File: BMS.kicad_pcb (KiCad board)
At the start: 2 copper layers, 2 parts, among them U1 ATtiny824-SSU, U2 TLV61070ADBV

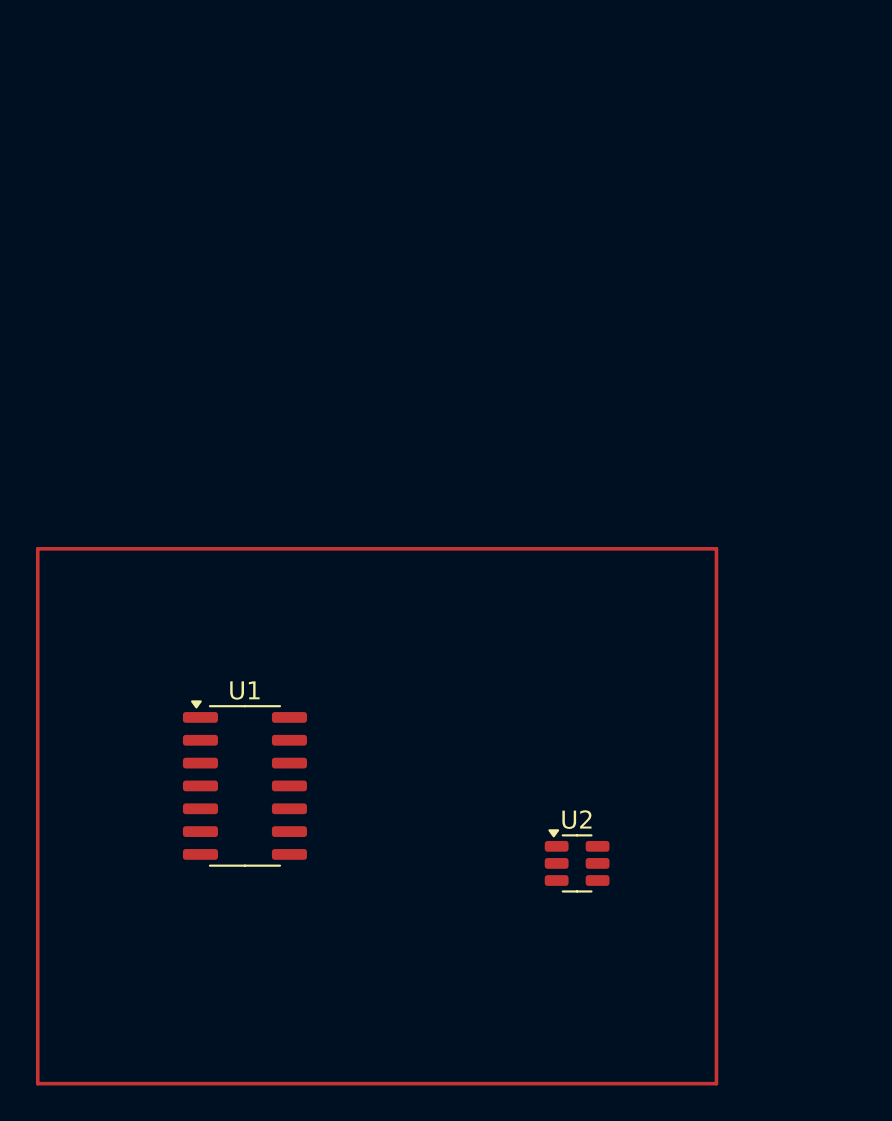
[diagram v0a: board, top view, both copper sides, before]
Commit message: Finished schematic
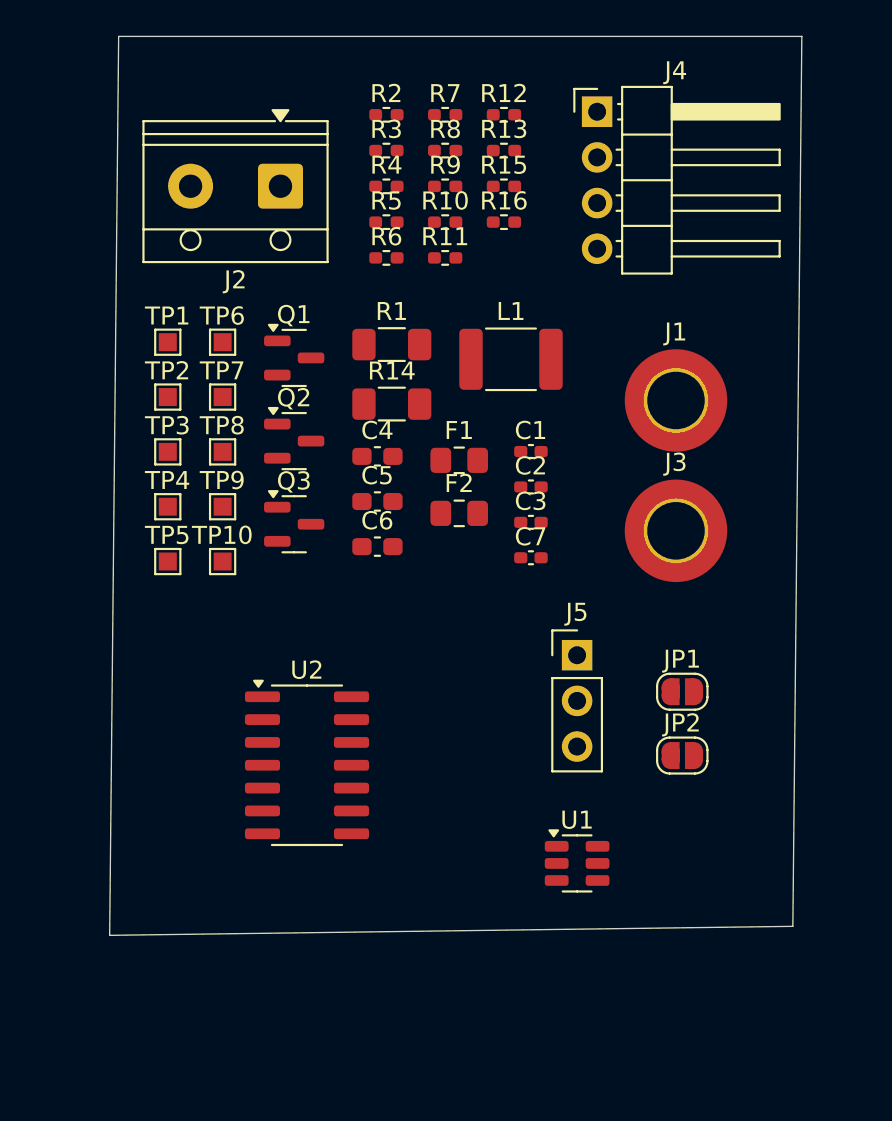
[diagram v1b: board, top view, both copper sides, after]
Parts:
- added C1: 100n, Capacitor_SMD:C_0402_1005Metric_Pad0.74x0.62mm_HandSolder, F.Cu at (150.4, 75.6)
- added C2: 100n, Capacitor_SMD:C_0402_1005Metric_Pad0.74x0.62mm_HandSolder, F.Cu at (150.4, 77.6)
- added C3: 100n, Capacitor_SMD:C_0402_1005Metric_Pad0.74x0.62mm_HandSolder, F.Cu at (150.4, 79.5)
- added C4: 10u, Capacitor_SMD:C_0603_1608Metric_Pad1.08x0.95mm_HandSolder, F.Cu at (141.9, 75.9)
- added C5: 10u, Capacitor_SMD:C_0603_1608Metric_Pad1.08x0.95mm_HandSolder, F.Cu at (141.9, 78.4)
- added C6: 10u, Capacitor_SMD:C_0603_1608Metric_Pad1.08x0.95mm_HandSolder, F.Cu at (141.9, 80.9)
- added C7: 270p, Capacitor_SMD:C_0402_1005Metric_Pad0.74x0.62mm_HandSolder, F.Cu at (150.4, 81.5)
- added F1: BSMD0805-110-6V, Fuse:Fuse_0805_2012Metric_Pad1.15x1.40mm_HandSolder, F.Cu at (146.4, 76.1)
- added F2: BSMD0805-110-6V, Fuse:Fuse_0805_2012Metric_Pad1.15x1.40mm_HandSolder, F.Cu at (146.4, 79.0)
- added J1: BATT+, MountingHole:MountingHole_3.2mm_M3_ISO7380_Pad_TopOnly, F.Cu at (158.5, 72.8)
- added J2: LOAD, TerminalBlock_RND:TerminalBlock_RND_205-00012_1x02_P5.00mm_Horizontal, F.Cu at (136.5, 60.8)
- added J3: BATT-, MountingHole:MountingHole_3.2mm_M3_ISO7380_Pad_TopOnly, F.Cu at (158.5, 80.0)
- added J4: QWIIC, Connector_PinHeader_2.54mm:PinHeader_1x04_P2.54mm_Horizontal, F.Cu at (154.1, 56.7)
- added J5: PROG, Connector_PinHeader_2.54mm:PinHeader_1x03_P2.54mm_Vertical, F.Cu at (153.0, 86.9)
- added JP1: MCU_VCC, Jumper:SolderJumper-2_P1.3mm_Open_RoundedPad1.0x1.5mm, F.Cu at (158.8, 89.0)
- added JP2: I2C_V, Jumper:SolderJumper-2_P1.3mm_Open_RoundedPad1.0x1.5mm, F.Cu at (158.8, 92.5)
- added L1: 2.2uH, Inductor_SMD:L_1812_4532Metric_Pad1.30x3.40mm_HandSolder, F.Cu at (149.3, 70.5)
- added Q1: SI2333, Package_TO_SOT_SMD:SOT-23, F.Cu at (137.3, 70.4)
- added Q2: SI2333, Package_TO_SOT_SMD:SOT-23, F.Cu at (137.3, 75.0)
- added Q3: SI2333, Package_TO_SOT_SMD:SOT-23, F.Cu at (137.3, 79.6)
- added R1: 0.1R, Resistor_SMD:R_1206_3216Metric_Pad1.30x1.75mm_HandSolder, F.Cu at (142.7, 69.6)
- added R10: 100k, Resistor_SMD:R_0402_1005Metric_Pad0.72x0.64mm_HandSolder, F.Cu at (145.7, 62.8)
- added R11: 120R, Resistor_SMD:R_0402_1005Metric_Pad0.72x0.64mm_HandSolder, F.Cu at (145.7, 64.8)
- added R12: 120R, Resistor_SMD:R_0402_1005Metric_Pad0.72x0.64mm_HandSolder, F.Cu at (148.9, 56.9)
- added R13: 1M, Resistor_SMD:R_0402_1005Metric_Pad0.72x0.64mm_HandSolder, F.Cu at (148.9, 58.9)
- added R14: 0.1R, Resistor_SMD:R_1206_3216Metric_Pad1.30x1.75mm_HandSolder, F.Cu at (142.7, 73.0)
- added R15: 120R, Resistor_SMD:R_0402_1005Metric_Pad0.72x0.64mm_HandSolder, F.Cu at (148.9, 60.8)
- added R16: 100k, Resistor_SMD:R_0402_1005Metric_Pad0.72x0.64mm_HandSolder, F.Cu at (148.9, 62.8)
- added R2: 1M, Resistor_SMD:R_0402_1005Metric_Pad0.72x0.64mm_HandSolder, F.Cu at (142.4, 56.9)
- added R3: 1M, Resistor_SMD:R_0402_1005Metric_Pad0.72x0.64mm_HandSolder, F.Cu at (142.4, 58.9)
- added R4: 1M, Resistor_SMD:R_0402_1005Metric_Pad0.72x0.64mm_HandSolder, F.Cu at (142.4, 60.8)
- added R5: 1M, Resistor_SMD:R_0402_1005Metric_Pad0.72x0.64mm_HandSolder, F.Cu at (142.4, 62.8)
- added R6: 1M, Resistor_SMD:R_0402_1005Metric_Pad0.72x0.64mm_HandSolder, F.Cu at (142.4, 64.8)
- added R7: 1M, Resistor_SMD:R_0402_1005Metric_Pad0.72x0.64mm_HandSolder, F.Cu at (145.7, 56.9)
- added R8: 1M, Resistor_SMD:R_0402_1005Metric_Pad0.72x0.64mm_HandSolder, F.Cu at (145.7, 58.9)
- added R9: 560k, Resistor_SMD:R_0402_1005Metric_Pad0.72x0.64mm_HandSolder, F.Cu at (145.7, 60.8)
- added TP1: TestPoint, TestPoint:TestPoint_Pad_1.0x1.0mm, F.Cu at (130.2, 69.5)
- added TP10: TestPoint, TestPoint:TestPoint_Pad_1.0x1.0mm, F.Cu at (133.3, 81.7)
- added TP2: TestPoint, TestPoint:TestPoint_Pad_1.0x1.0mm, F.Cu at (130.2, 72.6)
- added TP3: TestPoint, TestPoint:TestPoint_Pad_1.0x1.0mm, F.Cu at (130.2, 75.6)
- added TP4: TestPoint, TestPoint:TestPoint_Pad_1.0x1.0mm, F.Cu at (130.2, 78.7)
- added TP5: TestPoint, TestPoint:TestPoint_Pad_1.0x1.0mm, F.Cu at (130.2, 81.7)
- added TP6: TestPoint, TestPoint:TestPoint_Pad_1.0x1.0mm, F.Cu at (133.3, 69.5)
- added TP7: TestPoint, TestPoint:TestPoint_Pad_1.0x1.0mm, F.Cu at (133.3, 72.6)
- added TP8: TestPoint, TestPoint:TestPoint_Pad_1.0x1.0mm, F.Cu at (133.3, 75.6)
- added TP9: TestPoint, TestPoint:TestPoint_Pad_1.0x1.0mm, F.Cu at (133.3, 78.7)
- moved U2 3.64 mm to (138.0, 93.0)
- renumbered U2 to U1, U1 to U2
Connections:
- U1 pad 1: unconnected-(U2-SW-Pad1) -> Net-(U1-SW)
- U1 pad 2: unconnected-(U2-GND-Pad2) -> GND
- U1 pad 3: unconnected-(U2-EN-Pad3) -> Net-(JP1-B)
- U1 pad 4: unconnected-(U2-V_{FB}-Pad4) -> Net-(U1-V_{FB})
- U1 pad 5: unconnected-(U2-V_{OUT}-Pad5) -> VCC
- U1 pad 6: unconnected-(U2-V_{IN}-Pad6) -> Net-(JP1-B)
- U2 pad 1: unconnected-(U1-VCC-Pad1) -> VCC
- U2 pad 10: unconnected-(U1-~{RESET}/PA0-Pad10) -> UPDI
- U2 pad 11: unconnected-(U1-PA1-Pad11) -> ADC_SP
- U2 pad 12: unconnected-(U1-AIN2-Pad12) -> ADC_BATT
- U2 pad 13: unconnected-(U1-AIN3-Pad13) -> ADC_LOAD
- U2 pad 14: unconnected-(U1-GND-Pad14) -> GND
- U2 pad 2: unconnected-(U1-PA4-Pad2) -> CUTOFF
- U2 pad 3: unconnected-(U1-PA5-Pad3) -> Net-(U2-PA5)
- U2 pad 4: unconnected-(U1-AIN6-Pad4) -> ADC_LN
- U2 pad 5: unconnected-(U1-AIN7-Pad5) -> ADC_LP
- U2 pad 6: unconnected-(U1-RXD-Pad6) -> 3V3CUTOFF
- U2 pad 7: unconnected-(U1-TXD-Pad7) -> Net-(U2-TXD)
- U2 pad 8: unconnected-(U1-SDA-Pad8) -> SDA
- U2 pad 9: unconnected-(U1-SCL-Pad9) -> SCL
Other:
- board outline added: 38.5 x 50 mm

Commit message: First PCB design
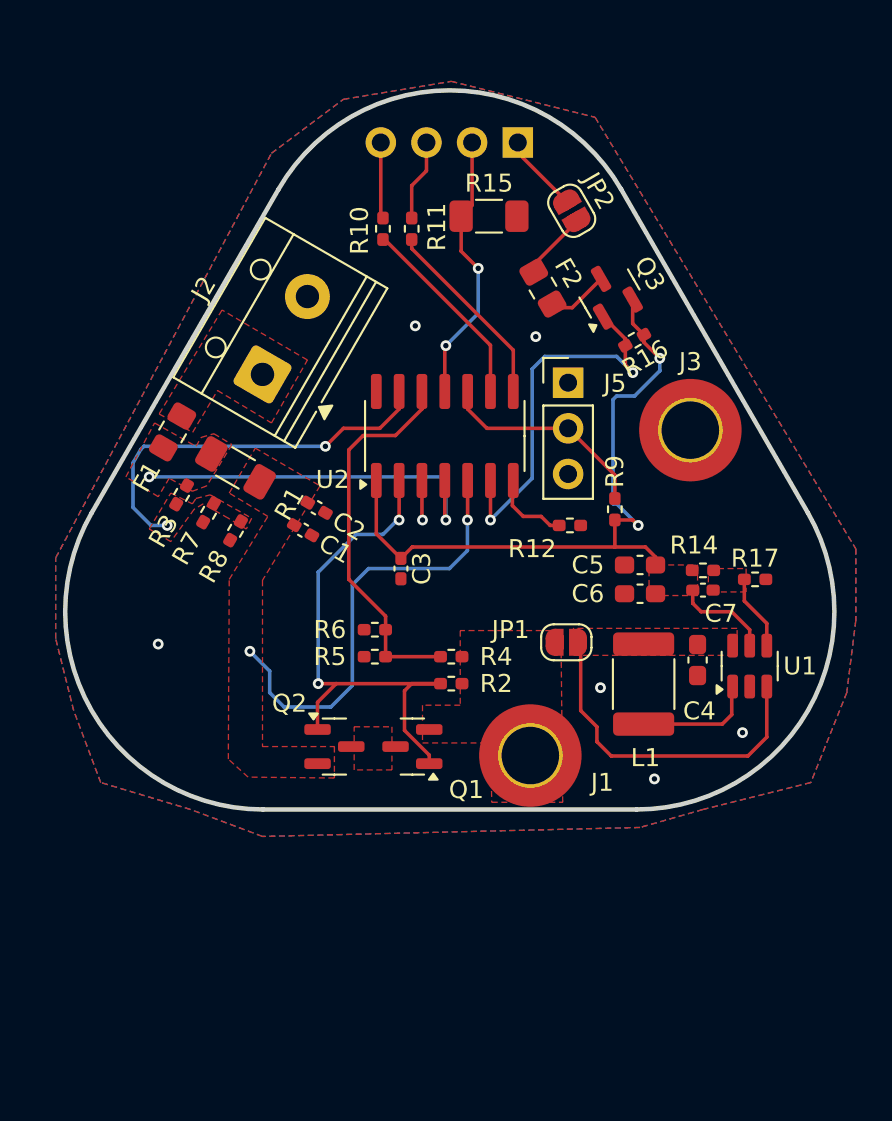
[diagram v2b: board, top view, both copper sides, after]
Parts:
- removed TP1, TP10, TP2, TP3, TP4, TP5, TP6, TP7, TP8, TP9: TestPoint, TestPoint:TestPoint_Pad_1.0x1.0mm
- J4: moved to B.Cu
- moved R2 31.8 mm to (146.0, 88.5), turned to 180 degrees
- moved JP2 30.9 mm to (152.7, 62.2), turned to -60 degrees
- moved R4 26.4 mm to (146.0, 87.0), turned to 180 degrees
- moved R17 26.3 mm to (162.9, 82.7)
- moved R7 25.8 mm to (132.5, 79.0), turned to -120 degrees
- moved R14 25.7 mm to (160.0, 82.2)
- moved R5 24.2 mm to (141.8, 87.0), turned to 180 degrees
- moved R8 24.2 mm to (134.0, 80.0), turned to -120 degrees
- moved Q1 22.6 mm to (143.8, 92.0), turned to 180 degrees
- moved R3 22.3 mm to (131.0, 78.0), turned to -120 degrees
- moved Q3 21.7 mm to (154.8, 66.8), turned to 120 degrees
- moved J1 21.3 mm to (150.4, 92.5)
- moved C4 21.1 mm to (159.7, 87.2), turned to -90 degrees
- moved R6 20.7 mm to (141.8, 85.5), turned to 180 degrees
- moved U2 19.9 mm to (145.6, 74.7), turned to 90 degrees
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- renumbered R12 to R10, R15 to R12, R9 to R14, R14 to R15, R13 to R16, R10 to R17, R16 to R9
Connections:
- J4 pad 1: ADC_SP -> Net-(J4-Pin_1)
- J4 pad 2: Net-(J4-Pin_2) -> ADC_SP
- JP2 pad 1: Net-(J4-Pin_2) -> Net-(J4-Pin_1)
- R10 pad 1: Net-(J4-Pin_3) -> Net-(J4-Pin_4)
- R10 pad 2: SDA -> SCL
- R11 pad 1: Net-(J4-Pin_4) -> Net-(J4-Pin_3)
- R11 pad 2: SCL -> SDA
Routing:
- net VCC: track 0.00 -> 43.9 mm, vias 0 -> 2
- net CUTOFF: track 0.00 -> 30.7 mm, vias 0 -> 2
- net ADC_LP: track 0.00 -> 24.9 mm, vias 0 -> 2
- net ADC_LOAD: track 0.00 -> 22.4 mm, vias 0 -> 2
- net 3V3CUTOFF: track 0.00 -> 21.6 mm, vias 0 -> 2
- net ADC_BATT: track 0.00 -> 21.4 mm
- net ADC_LN: track 0.00 -> 20.9 mm, vias 0 -> 2
- net Net-(JP1-B): track 0.00 -> 18.4 mm
- net ADC_SP: track 0.00 -> 15.7 mm, vias 0 -> 2
- net UPDI: track 0.00 -> 12.0 mm
- net SCL: track 0.00 -> 11.0 mm
- net SDA: track 0.00 -> 10.9 mm
- net Net-(U1-SW): track 0.00 -> 6.70 mm
- net Net-(J4-Pin_3): track 0.00 -> 4.54 mm
- net Net-(U2-TXD): track 0.00 -> 4.48 mm
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- added copper zone on F.Cu, net +BATT
- added copper zone on F.Cu, net ADC_LN
- added copper zone on F.Cu, net ADC_LOAD
- added copper zone on F.Cu, net ADC_LP
- added copper zone on B.Cu, net GND
- added copper zone on F.Cu, net GND
- added copper zone on F.Cu, net Net-(J2-Pin_1)
- added copper zone on F.Cu, net Net-(JP1-B)
- added copper zone on F.Cu, net Net-(Q1-D)
- added copper zone on F.Cu, net Net-(U1-V_{FB})
- added copper zone on F.Cu, net VCC
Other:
- board size 38.5 x 50 mm -> 42.8 x 40 mm
